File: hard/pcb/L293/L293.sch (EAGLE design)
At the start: 15 parts, among them IC1 L293DD

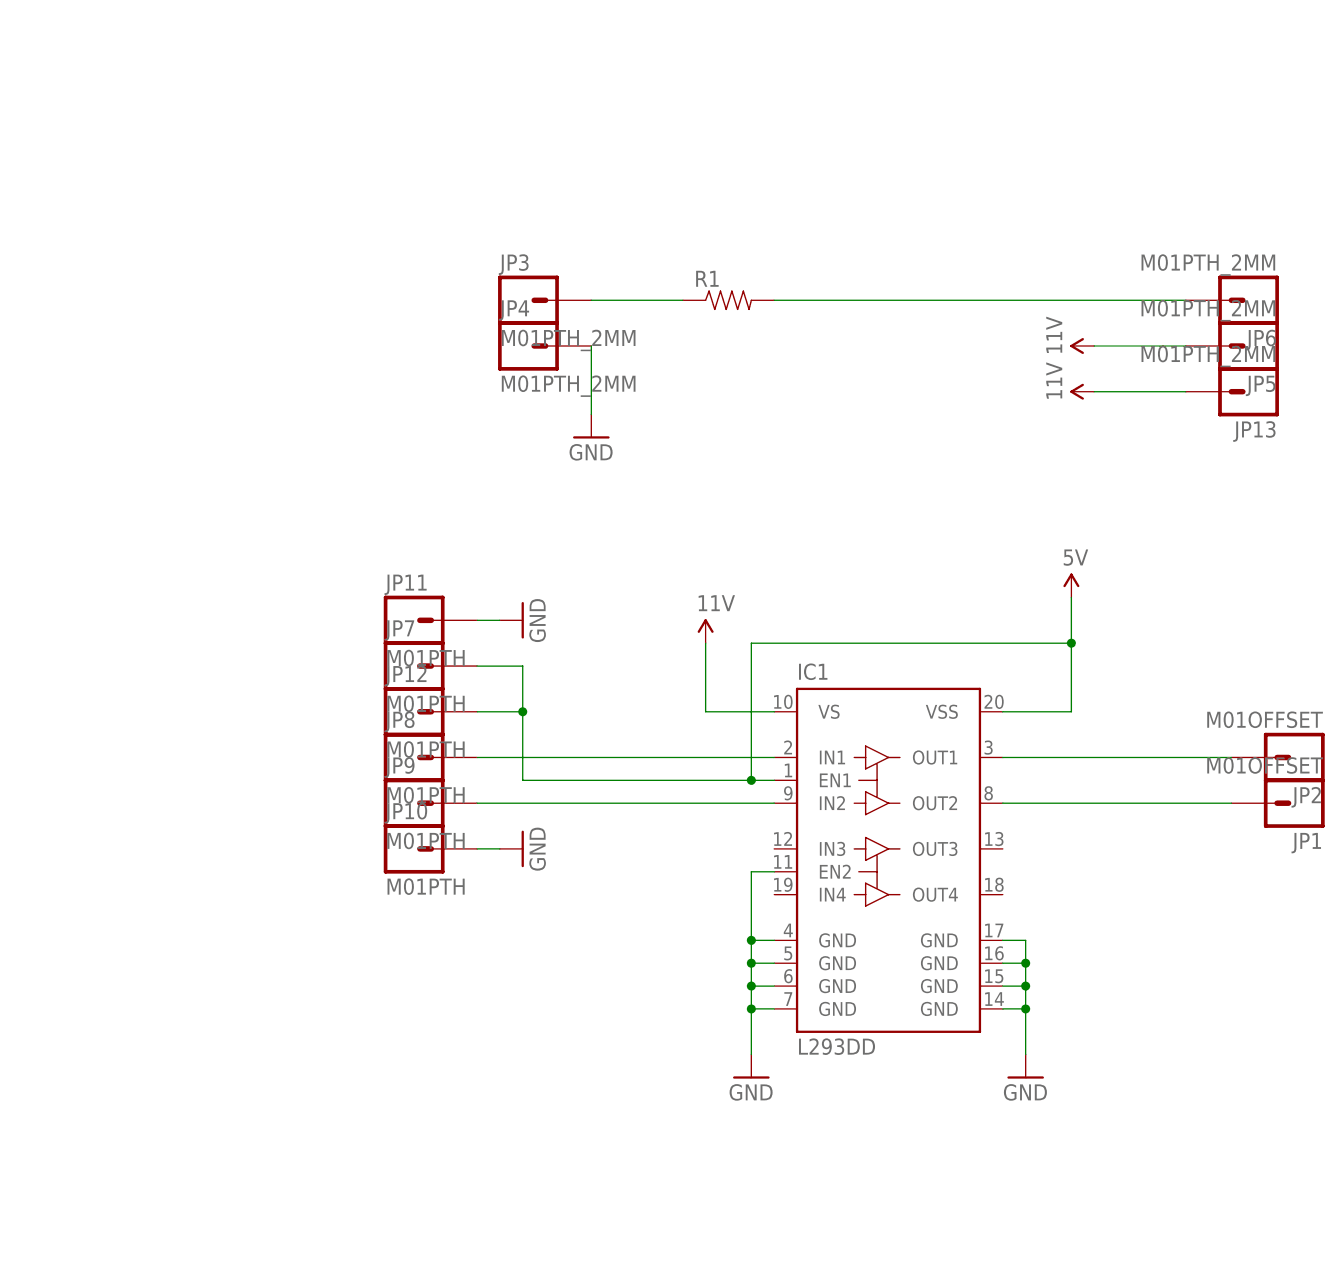
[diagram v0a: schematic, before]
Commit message: L239 rework
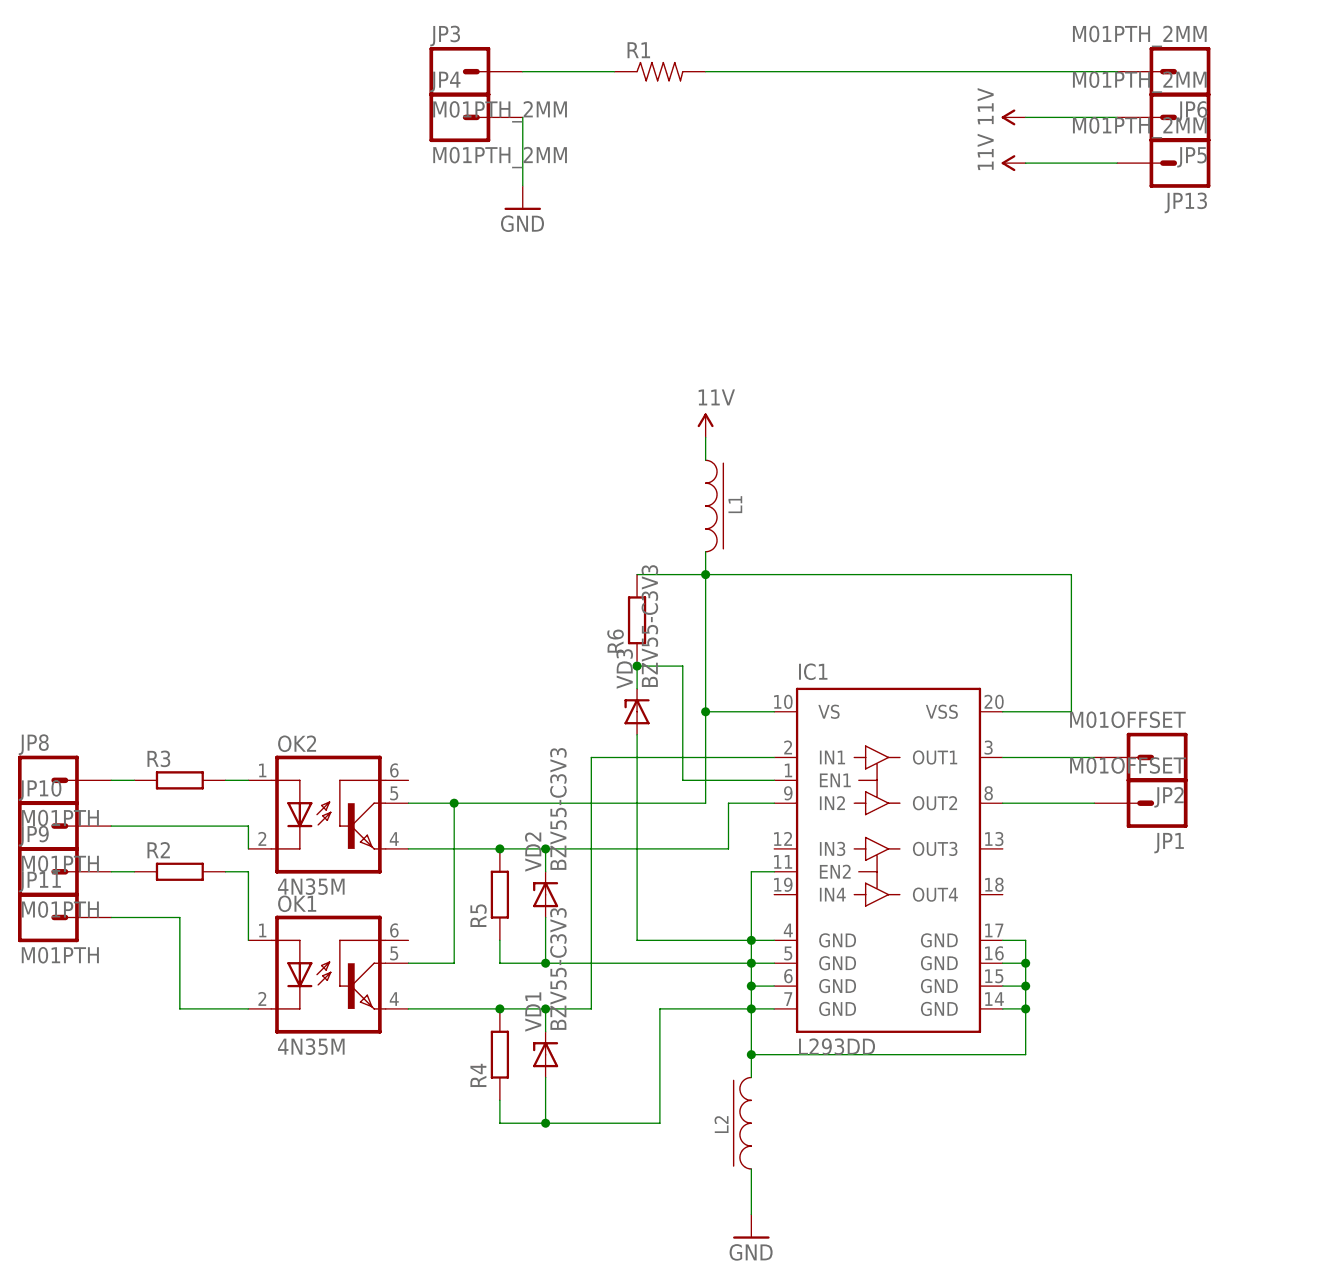
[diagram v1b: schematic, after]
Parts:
- removed JP12, JP7: M01PTH, SparkFun-Connectors:M01PTH
- added L1, L2: (no value), inductor-cooper:DRA127
- added OK1, OK2: 4N35M, optocoupler:4N35M
- added R2, R3, R4, R5, R6: (no value), barthess:RESISTOR0805
- added VD1, VD2, VD3: BZV55-C3V3, barthess:BZV55-C3V3
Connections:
- removed net 5V: IC1.EN1, IC1.VSS, JP12.1, JP7.1
- new net GND_DIRT: IC1.EN2, IC1.GND@1, IC1.GND@2, IC1.GND@3, IC1.GND@4, IC1.GND@5, IC1.GND@6, IC1.GND@7, IC1.GND@8, L2.2, R4.1, R5.1, VD1.A, VD2.A, VD3.A
- new net N$10: OK1.A, R2.2
- new net N$11: JP11.1, OK1.C
- new net N$12: JP10.1, OK2.C
- new net N$13: OK2.A, R3.2
- new net N$14: IC1.EN1, R6.1, VD3.C
- new net N$15: IC1.IN2, OK2.EMI, R5.2, VD2.C
- new net N$17: IC1.IN1, OK1.EMI, R4.2, VD1.C
- new net N$9: IC1.VS, IC1.VSS, L1.2, OK1.COL, OK2.COL, R6.2
- net 1.0V: now also L1.1; no longer IC1.VS
- net GND: now also L2.1; no longer IC1.EN2, IC1.GND@1, IC1.GND@2, IC1.GND@3, IC1.GND@4, IC1.GND@5, IC1.GND@6, IC1.GND@7, IC1.GND@8, JP10.1, JP11.1
- net N$7: now also R2.1; no longer IC1.IN2
- net N$8: now also R3.1; no longer IC1.IN1
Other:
- moved on the sheet: JP1, JP10, JP11, JP13, JP2, JP3, JP4, JP5, JP6, JP8, JP9, R1
